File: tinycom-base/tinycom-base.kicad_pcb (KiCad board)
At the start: 2 copper layers, 45.2 x 45.2 mm, 38 parts, among them J1 MICRO_SD_HINGE, P1 CONN_02X08, P2 CONN_02X08, P3 USB_A, P4 USB_B, U1 SY8008BAAC, U2 SY8008BAAC, U3 SY8008BAAC

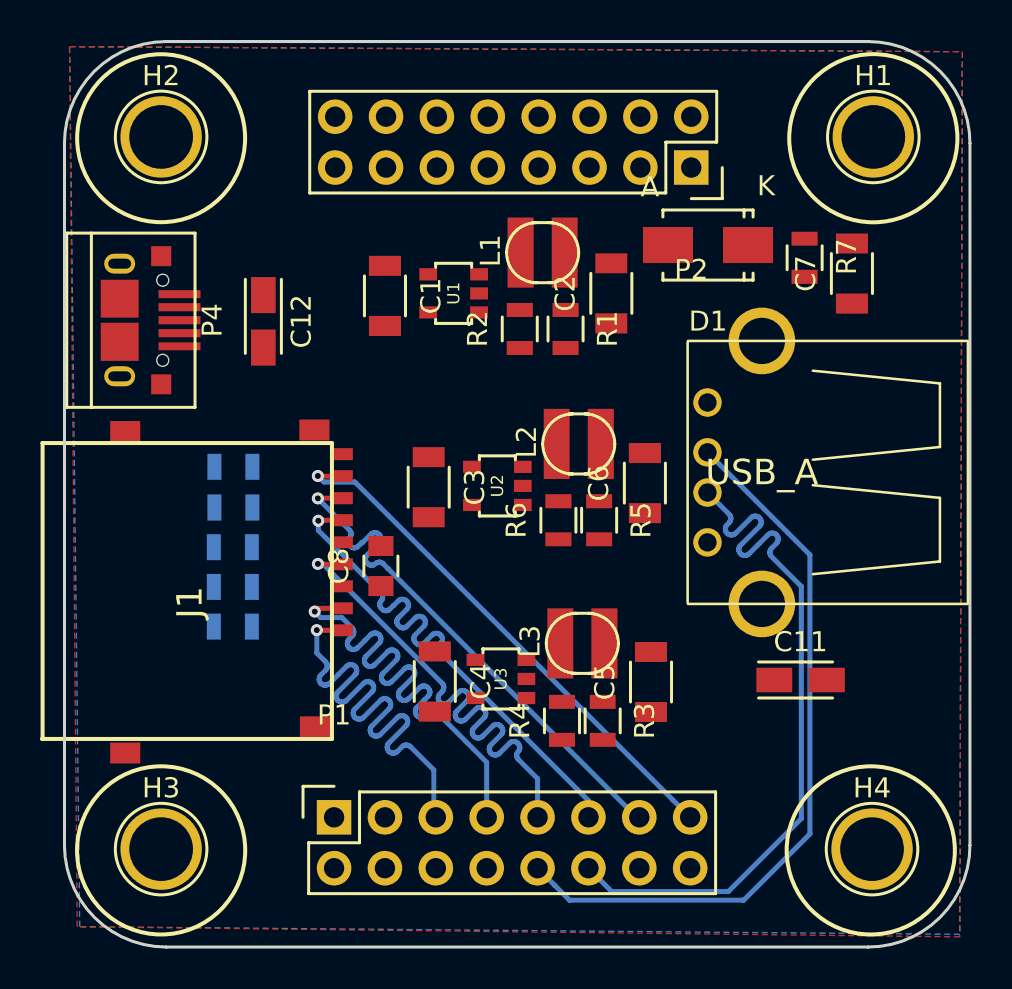
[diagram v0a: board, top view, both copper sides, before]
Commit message: done update base board
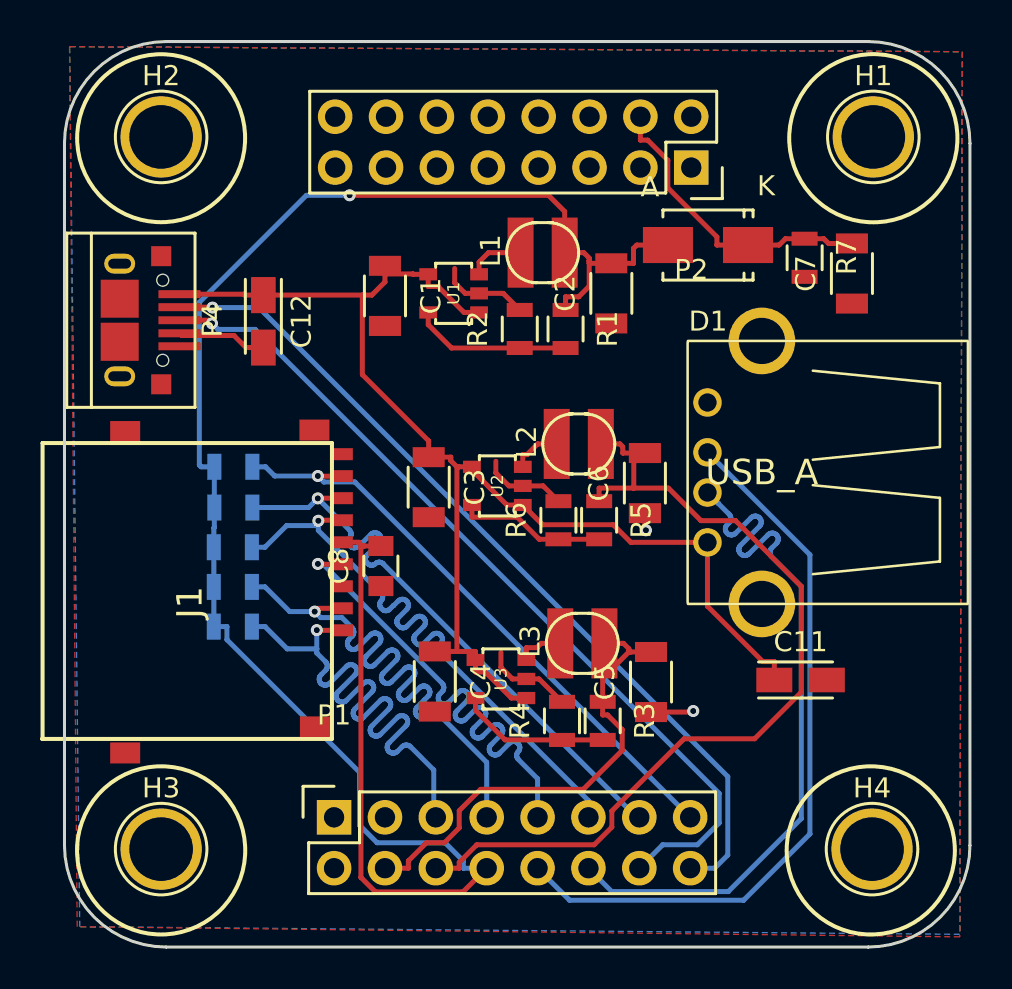
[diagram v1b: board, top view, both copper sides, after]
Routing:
- net VCC_33: track 0.00 -> 95.8 mm, vias 0 -> 1
- net +5V: track 0.00 -> 66.6 mm
- net VCC_14: track 0.00 -> 44.9 mm
- net UDM0: track 0.00 -> 43.2 mm, vias 0 -> 1
- net UDP0: track 0.00 -> 43.1 mm, vias 0 -> 1
- net VCC_15: track 0.00 -> 23.6 mm
- net GND: track 0.00 -> 20.8 mm, vias 0 -> 2
- net VCC_30: track 0.00 -> 15.2 mm
- net Net-(R1-Pad2): track 0.00 -> 7.95 mm
- net Net-(R3-Pad2): track 0.00 -> 7.57 mm
- net Net-(R5-Pad2): track 0.00 -> 7.42 mm
- net SDC0_CMD: track 26.8 -> 30.6 mm
- net SDC0_D1: track 26.8 -> 30.5 mm
- net SDC0_D0: track 26.8 -> 30.5 mm
- net SDC0_D3: track 26.9 -> 30.3 mm
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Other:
- net class Default: clearance 0.18 -> 0.15
- rule trace_clearance: 0.18 -> 0.15
